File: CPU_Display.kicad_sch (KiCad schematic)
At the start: 1 part

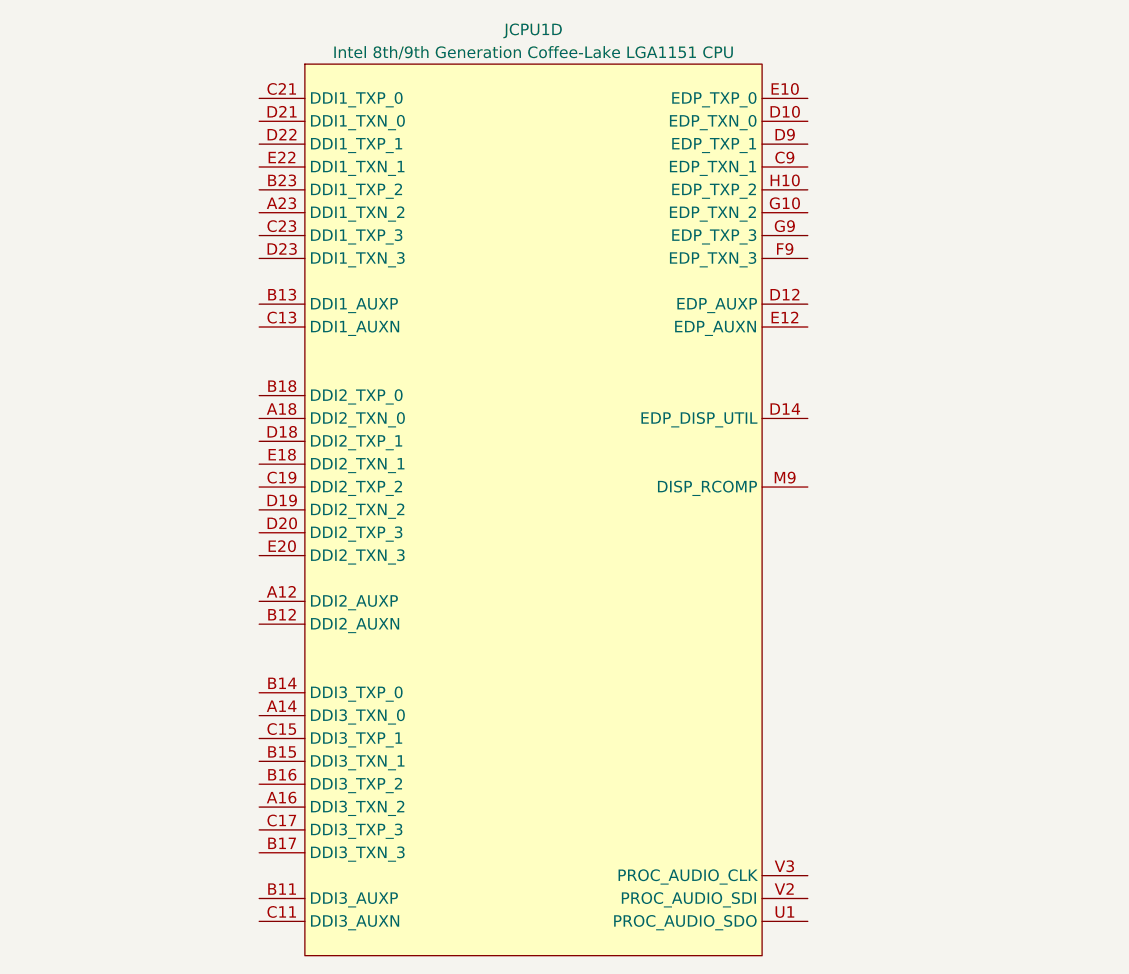
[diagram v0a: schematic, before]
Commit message: Some DP and power work
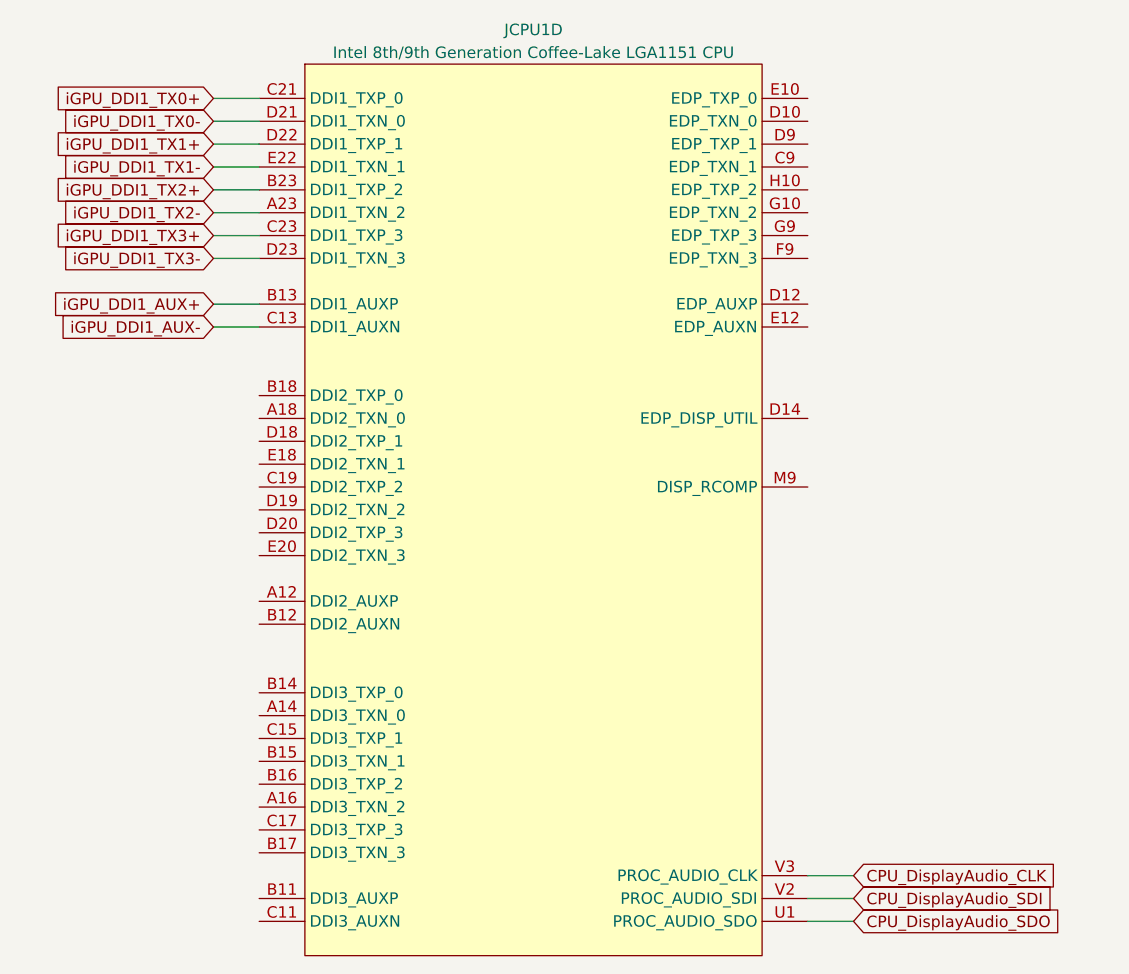
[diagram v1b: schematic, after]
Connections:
- net iGPU_DDI1_TX2-: now reaches JCPU1.A23 (DDI1_TXN_2)
- net iGPU_DDI1_AUX+: now reaches JCPU1.B13 (DDI1_AUXP)
- net iGPU_DDI1_TX2+: now reaches JCPU1.B23 (DDI1_TXP_2)
- net iGPU_DDI1_AUX-: now reaches JCPU1.C13 (DDI1_AUXN)
- net iGPU_DDI1_TX0+: now reaches JCPU1.C21 (DDI1_TXP_0)
- net iGPU_DDI1_TX3+: now reaches JCPU1.C23 (DDI1_TXP_3)
- net iGPU_DDI1_TX0-: now reaches JCPU1.D21 (DDI1_TXN_0)
- net iGPU_DDI1_TX1+: now reaches JCPU1.D22 (DDI1_TXP_1)
- net iGPU_DDI1_TX3-: now reaches JCPU1.D23 (DDI1_TXN_3)
- net iGPU_DDI1_TX1-: now reaches JCPU1.E22 (DDI1_TXN_1)
- net CPU_DisplayAudio_SDO: now reaches JCPU1.U1 (PROC_AUDIO_SDO)
- net CPU_DisplayAudio_SDI: now reaches JCPU1.V2 (PROC_AUDIO_SDI)
- net CPU_DisplayAudio_CLK: now reaches JCPU1.V3 (PROC_AUDIO_CLK)

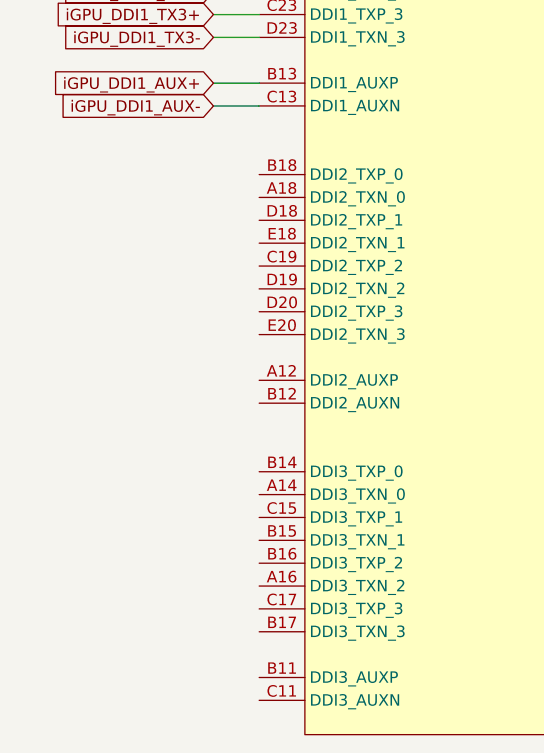
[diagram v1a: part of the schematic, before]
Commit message: More DP
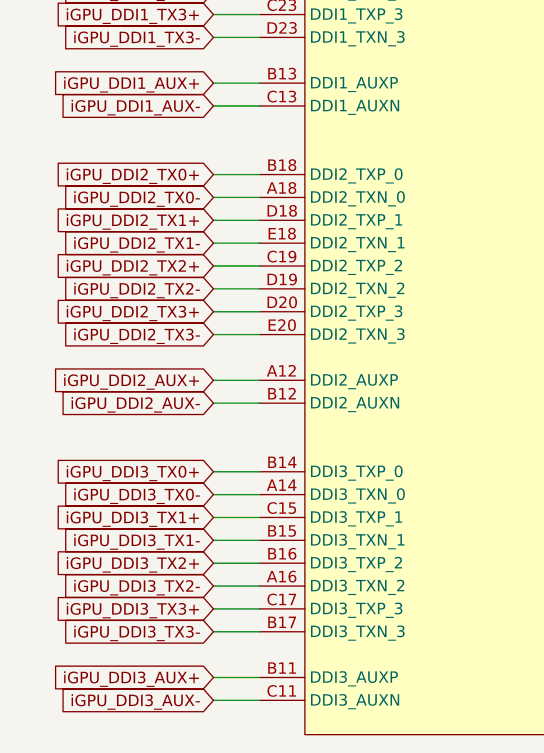
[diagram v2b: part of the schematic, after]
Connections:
- net iGPU_DDI2_AUX+: now reaches JCPU1.A12 (DDI2_AUXP)
- net iGPU_DDI3_TX0-: now reaches JCPU1.A14 (DDI3_TXN_0)
- net iGPU_DDI3_TX2-: now reaches JCPU1.A16 (DDI3_TXN_2)
- net iGPU_DDI2_TX0-: now reaches JCPU1.A18 (DDI2_TXN_0)
- net iGPU_DDI3_AUX+: now reaches JCPU1.B11 (DDI3_AUXP)
- net iGPU_DDI2_AUX-: now reaches JCPU1.B12 (DDI2_AUXN)
- net iGPU_DDI3_TX0+: now reaches JCPU1.B14 (DDI3_TXP_0)
- net iGPU_DDI3_TX1-: now reaches JCPU1.B15 (DDI3_TXN_1)
- net iGPU_DDI3_TX2+: now reaches JCPU1.B16 (DDI3_TXP_2)
- net iGPU_DDI3_TX3-: now reaches JCPU1.B17 (DDI3_TXN_3)
- net iGPU_DDI2_TX0+: now reaches JCPU1.B18 (DDI2_TXP_0)
- net iGPU_DDI3_AUX-: now reaches JCPU1.C11 (DDI3_AUXN)
- net iGPU_DDI3_TX1+: now reaches JCPU1.C15 (DDI3_TXP_1)
- net iGPU_DDI3_TX3+: now reaches JCPU1.C17 (DDI3_TXP_3)
- net iGPU_DDI2_TX2+: now reaches JCPU1.C19 (DDI2_TXP_2)
- net iGPU_DDI2_TX1+: now reaches JCPU1.D18 (DDI2_TXP_1)
- net iGPU_DDI2_TX2-: now reaches JCPU1.D19 (DDI2_TXN_2)
- net iGPU_DDI2_TX3+: now reaches JCPU1.D20 (DDI2_TXP_3)
- net iGPU_DDI2_TX1-: now reaches JCPU1.E18 (DDI2_TXN_1)
- net iGPU_DDI2_TX3-: now reaches JCPU1.E20 (DDI2_TXN_3)
